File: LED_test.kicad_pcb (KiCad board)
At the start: 2 copper layers, 100 x 100 mm, 79 parts, among them J1 Conn_01x08_Male, J2 Conn_01x09_Male, Q1 FDC6330L, Q2 DMN6075S, U1 MAX14662, U2 MAX1978, U3 DAC081C085, U4 ADC101C021CIMM, U5 REF3333, U6 LTC1669IMS8, U7 AD8603, U8 PAC1931

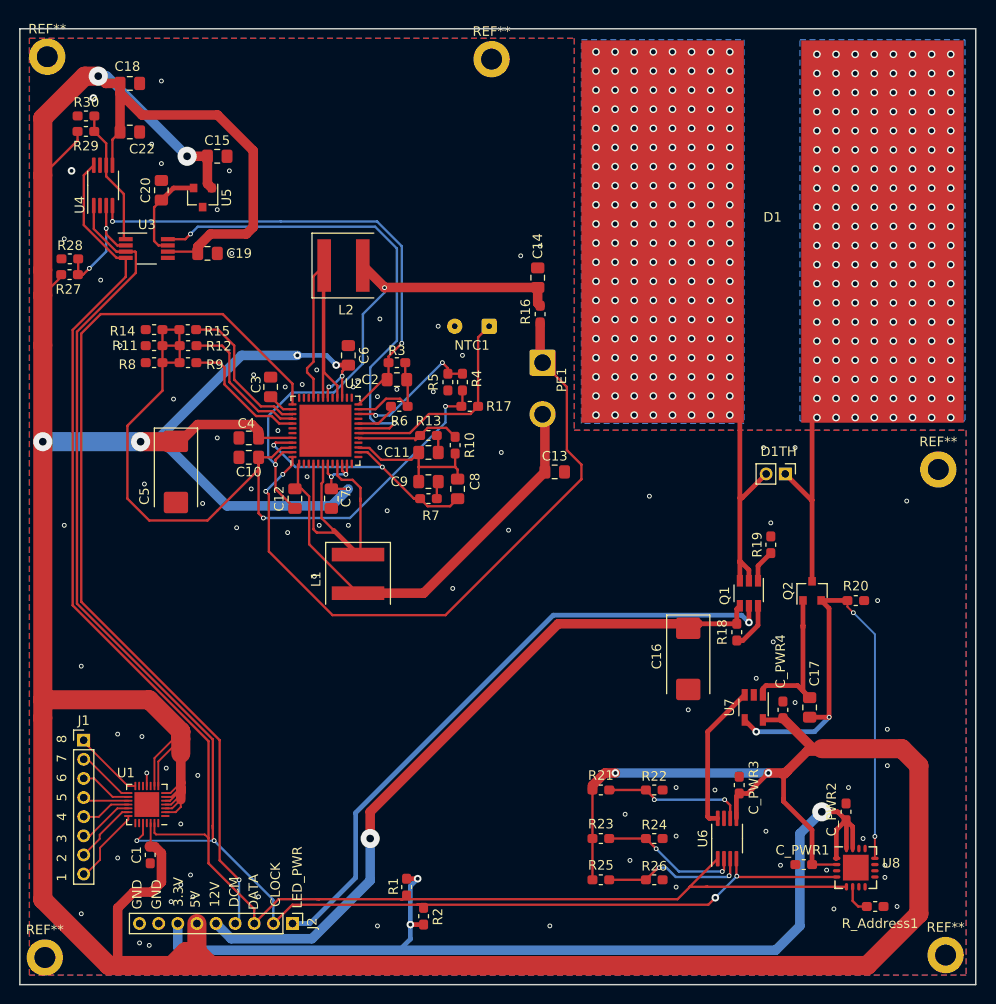
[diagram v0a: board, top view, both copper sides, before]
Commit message: Current PCB
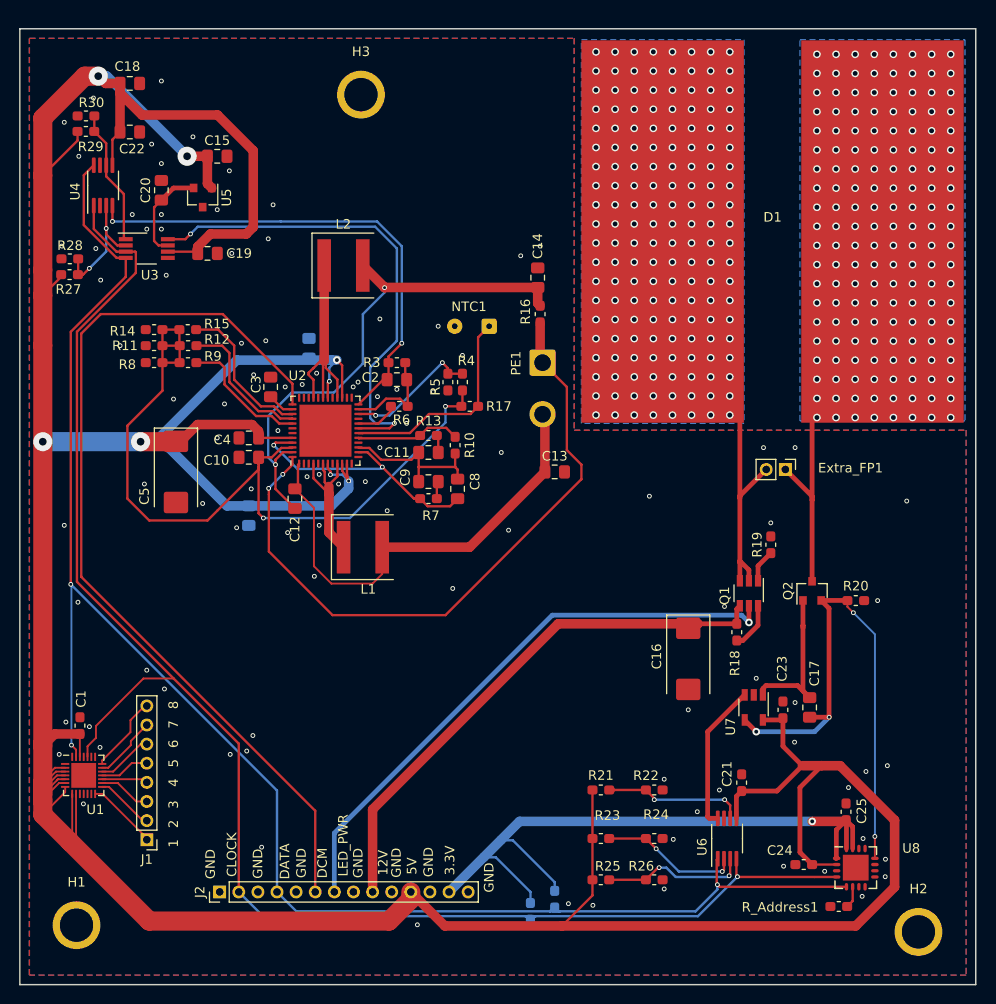
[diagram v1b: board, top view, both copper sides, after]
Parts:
- removed D1TH: PinHeader_1x02_P2.00mm_Vertical, Connector_PinHeader_2.00mm:PinHeader_1x02_P2.00mm_Vertical
- removed REF** (x5): MountingHole_2.2mm_M2_DIN965_Pad, MountingHole:MountingHole_2.2mm_M2_DIN965_Pad
- added Extra_FP1: LED, Connector_PinHeader_2.00mm:PinHeader_1x02_P2.00mm_Vertical, F.Cu at (180.1, 86.1)
- added H1: MountingHole, MountingHole:MountingHole_3.5mm_Pad, F.Cu at (105.9, 133.8)
- added H2: MountingHole, MountingHole:MountingHole_3.5mm_Pad, F.Cu at (194.0, 134.5)
- added H3: MountingHole, MountingHole:MountingHole_3.5mm_Pad, F.Cu at (135.7, 46.9)
- C6, C7, R1, R2: moved to B.Cu
- J2: value Conn_01x09_Male -> Conn_01x14_Male; footprint Connector_PinHeader_2.00mm:PinHeader_1x09_P2.00mm_Vertical -> Connector_PinHeader_2.00mm:PinHeader_1x14_P2.00mm_Vertical
- moved R1 15.5 mm to (156.0, 131.1)
- moved C1 15.4 mm to (106.3, 112.9), turned to 270 degrees
- moved J1 12.3 mm to (113.3, 124.8), turned to 180 degrees
- moved R2 11.2 mm to (153.4, 132.3), turned to 270 degrees
- moved C7 8.82 mm to (124.0, 90.9)
- moved J2 8.30 mm to (120.9, 130.3), turned to 90 degrees
- moved U1 7.27 mm to (106.7, 118.1), turned to 0 degrees
- moved C6 4.18 mm to (130.2, 73.4)
- moved R_Address1 3.81 mm to (185.7, 131.8), turned to 180 degrees
- moved L1 2.84 mm to (135.9, 94.2), turned to 0 degrees
- moved C21 0.36 mm to (175.5, 118.9)
- renumbered C_PWR3 to C21, C_PWR4 to C23, C_PWR1 to C24, C_PWR2 to C25
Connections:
- J2 pad 1: /LED2/LED_Power -> GND
- J2 pad 3: /Sheet5F1EB17F/DATA -> GND
- J2 pad 4: /Sheet5F1EB17F/DC_Current_Monitor -> /Sheet5F1EB17F/DATA
- J2 pad 5: +12V -> GND
- J2 pad 6: +5V -> /Sheet5F1EB17F/DC_Current_Monitor
- J2 pad 7: +3V3 -> /LED2/LED_Power
- J2 pad 9: GND -> +12V
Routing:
- net +5V: track 522.3 -> 450.8 mm, vias 13 -> 8
- net +3V3: track 106.1 -> 71.3 mm, vias 3 -> 1
- net Net-(L2-Pad1): track 43.1 -> 23.4 mm
- net +12V: track 76.4 -> 58.2 mm, vias 1 -> 0
- net Net-(L1-Pad1): track 32.2 -> 16.2 mm
- net /LED2/LED_Power: track 67.2 -> 61.0 mm
- net /Sheet5F1EB17F/DATA: track 169.0 -> 175.1 mm, vias 0 -> 3
- net /Sheet5F1EB17F/CLOCK: track 163.6 -> 166.7 mm, vias 4 -> 1
- net GND: track 1.79 -> 0.02 mm, vias 88 -> 99
- net Net-(C12-Pad2): track 47.8 -> 49.3 mm
- net Net-(R_Address1-Pad1): track 3.21 -> 2.30 mm
- net Net-(R10-Pad2): track 11.7 -> 11.0 mm
- net /Sheet5F1EB17F/DC_Current_Monitor: track 96.8 -> 96.7 mm, vias 1 -> 0
